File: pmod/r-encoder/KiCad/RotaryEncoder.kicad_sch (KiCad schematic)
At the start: 15 parts, among them J1 Conn_01x06, U1 PEC11R-4325F-S0012

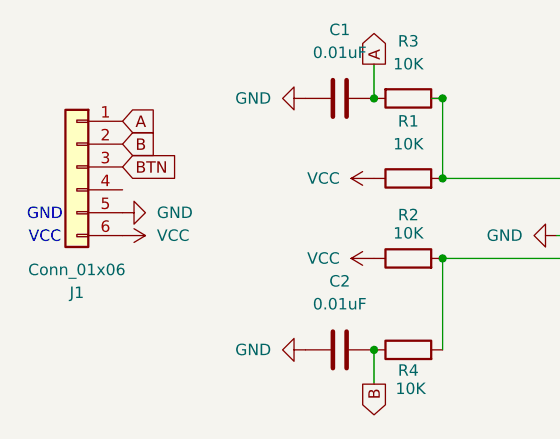
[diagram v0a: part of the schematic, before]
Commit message: fix: connectors
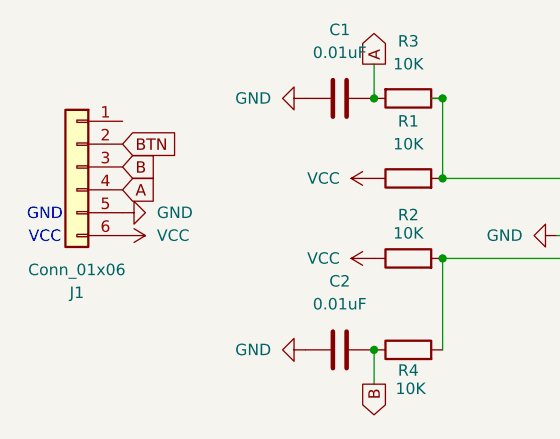
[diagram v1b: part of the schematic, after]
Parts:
- J1: footprint Connector_PinHeader_2.54mm:PinHeader_1x06_P2.54mm_Vertical -> Connector_PinHeader_2.54mm:PinHeader_1x06_P2.54mm_Horizontal
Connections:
- net A: now also J1.4 (Pin_4); no longer J1.1 (Pin_1)
- net B: now also J1.3 (Pin_3); no longer J1.2 (Pin_2)
- net BTN: now also J1.2 (Pin_2); no longer J1.3 (Pin_3)
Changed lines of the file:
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@@
-		)
-	)
-	(global_label "A"
-		(shape input)
-		(at 27.94 44.45 0)
-		(fields_autoplaced yes)
-		(effects
-			(font
-				(size 1.27 1.27)
-			)
-			(justify left)
-		)
-		(property "Intersheetrefs" "${INTERSHEET_REFS}"
-			(at 32.0138 44.45 0)
-			(effects
-				(font
-					(size 1.27 1.27)
-				)
-				(justify left)
-				(hide yes)
-			)
 		)
 	)
 	(global_label "B"
 		(shape input)
-		(at 27.94 46.99 0)
+		(at 27.94 49.53 0)
 		(fields_autoplaced yes)
 		(effects
@@
 		)
 		(property "Intersheetrefs" "${INTERSHEET_REFS}"
-			(at 32.1952 46.99 0)
+			(at 32.1952 49.53 0)
 			(effects
 				(font
@@
 	(global_label "BTN"
 		(shape input)
-		(at 27.94 49.53 0)
+		(at 27.94 46.99 0)
 		(fields_autoplaced yes)
 		(effects
@@
 		)
 		(property "Intersheetrefs" "${INTERSHEET_REFS}"
-			(at 34.4933 49.53 0)
+			(at 34.4933 46.99 0)
 			(effects
 				(font
@@
 				)
 				(justify right)
+				(hide yes)
+			)
+		)
+	)
+	(global_label "A"
+		(shape input)
+		(at 27.94 52.07 0)
+		(fields_autoplaced yes)
+		(effects
+			(font
+				(size 1.27 1.27)
+			)
+			(justify left)
+		)
+		(property "Intersheetrefs" "${INTERSHEET_REFS}"
+			(at 32.0138 52.07 0)
+			(effects
+				(font
+					(size 1.27 1.27)
+				)
+				(justify left)
 				(hide yes)
 			)
@@
 			)
 		)
-		(property "Footprint" "Connector_PinHeader_2.54mm:PinHeader_1x06_P2.54mm_Vertical"
+		(property "Footprint" "Connector_PinHeader_2.54mm:PinHeader_1x06_P2.54mm_Horizontal"
 			(at 22.86 49.53 0)
 			(effects
